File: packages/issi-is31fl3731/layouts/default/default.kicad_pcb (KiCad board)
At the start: 2 copper layers, 11 parts

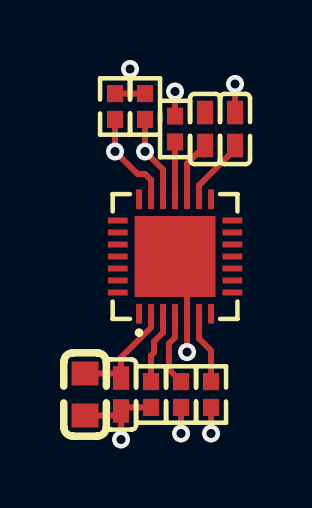
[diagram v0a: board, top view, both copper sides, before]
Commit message: fix some more packages
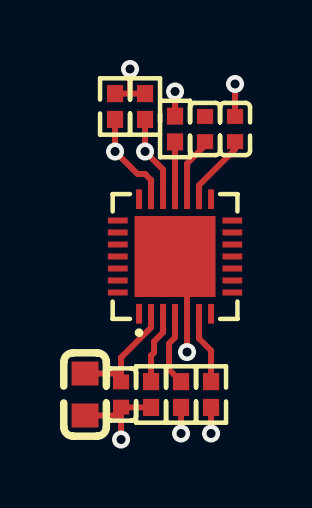
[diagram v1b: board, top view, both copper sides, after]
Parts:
- C1, C4, C5: value 100nF ±10% 16V X7R -> {8.99999998509884e-08..1.1000000014901162e-07}F
- C2: value 10µF ±20% 6.3V X5R -> {8.999999985098837e-06..1.1000000014901161e-05}F
- R1: value 20kΩ ±1% 62.5mW -> {20000.0±1.0%}Ω
- R2, R3, R6: value 10kΩ ±1% 62.5mW -> {10000.0±1.0%}Ω
- R4, R5: value 10kΩ ±1% 62.5mW -> {4700.0±1.0%}Ω
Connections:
- net CA1 renamed 21
- net CA2 renamed 22
- net CA3 renamed 23
- net CA4 renamed 24
- net CA5 renamed 25
- net CA6 renamed 26
- net CA7 renamed 27
- net CA8 renamed 28
- net CA9 renamed 1
- net CB1 renamed 7
- net CB2 renamed 8
- net CB3 renamed 9
- net CB4 renamed 10
- net CB5 renamed 11
- net CB6 renamed 12
- net CB7 renamed 13
- net CB8 renamed 14
- net CB9 renamed 15
- net GND renamed filter_capacitor-power-lv
- net IN renamed audio_input_capacitor-power-lv
- net VCC renamed hv
